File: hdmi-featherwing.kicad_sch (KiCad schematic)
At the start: 10 parts, among them J1 HDMI_A

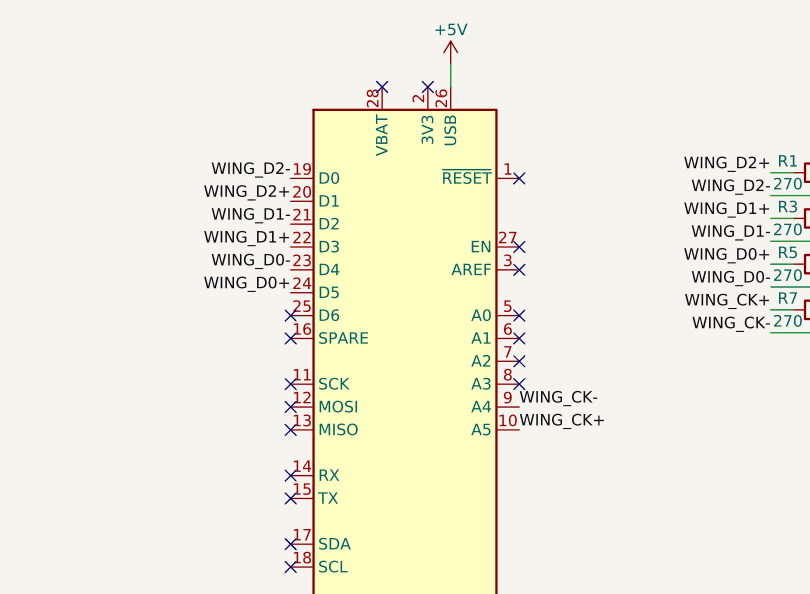
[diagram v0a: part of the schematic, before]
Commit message: route diffpairs
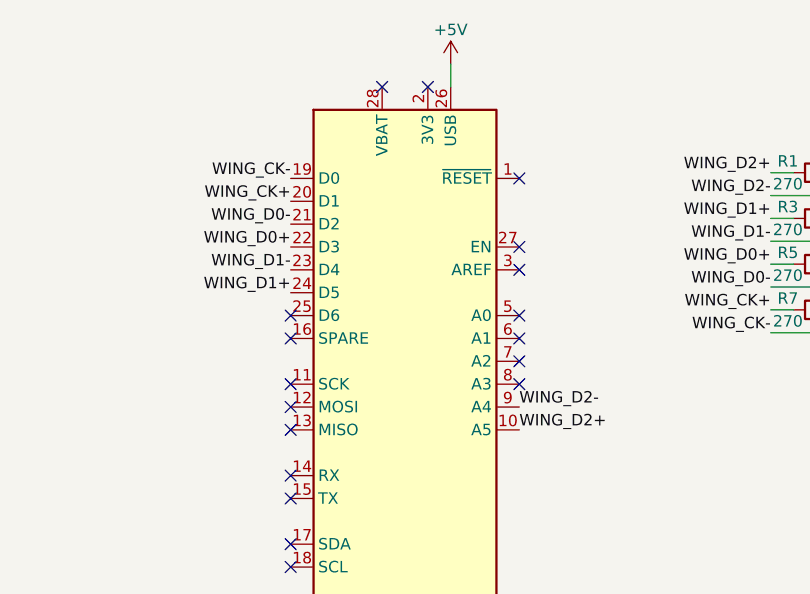
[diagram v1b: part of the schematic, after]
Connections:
- net WING_CK+: now also A1.20 (D1); no longer A1.10 (A5)
- net WING_CK-: now also A1.19 (D0); no longer A1.9 (A4)
- net WING_D0+: now also A1.22 (D3); no longer A1.24 (D5)
- net WING_D0-: now also A1.21 (D2); no longer A1.23 (D4)
- net WING_D1+: now also A1.24 (D5); no longer A1.22 (D3)
- net WING_D1-: now also A1.23 (D4); no longer A1.21 (D2)
- net WING_D2+: now also A1.10 (A5); no longer A1.20 (D1)
- net WING_D2-: now also A1.9 (A4); no longer A1.19 (D0)
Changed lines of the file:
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@@
     (stroke (width 0) (type solid) (color 0 0 0 0))
   )
-  (label "WING_D2-" (at 97.79 62.865 180)
+  (label "WING_CK-" (at 97.79 62.865 180)
     (effects (font (size 1.27 1.27)) (justify right bottom))
   )
-  (label "WING_D2+" (at 97.79 65.405 180)
+  (label "WING_CK+" (at 97.79 65.405 180)
     (effects (font (size 1.27 1.27)) (justify right bottom))
   )
-  (label "WING_D1-" (at 97.79 67.945 180)
+  (label "WING_D0-" (at 97.79 67.945 180)
     (effects (font (size 1.27 1.27)) (justify right bottom))
   )
-  (label "WING_D1+" (at 97.79 70.485 180)
+  (label "WING_D0+" (at 97.79 70.485 180)
     (effects (font (size 1.27 1.27)) (justify right bottom))
   )
-  (label "WING_D0-" (at 97.79 73.025 180)
+  (label "WING_D1-" (at 97.79 73.025 180)
     (effects (font (size 1.27 1.27)) (justify right bottom))
   )
-  (label "WING_D0+" (at 97.79 75.565 180)
+  (label "WING_D1+" (at 97.79 75.565 180)
     (effects (font (size 1.27 1.27)) (justify right bottom))
   )
-  (label "WING_CK-" (at 123.19 88.265 0)
+  (label "WING_D2-" (at 123.19 88.265 0)
     (effects (font (size 1.27 1.27)) (justify left bottom))
   )
-  (label "WING_CK+" (at 123.19 90.805 0)
+  (label "WING_D2+" (at 123.19 90.805 0)
     (effects (font (size 1.27 1.27)) (justify left bottom))
   )
